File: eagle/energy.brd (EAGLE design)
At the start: 51.7 x 57.8 mm, 19 parts, among them J1 S0, J2 NPN, T1 BC547, X1 P1

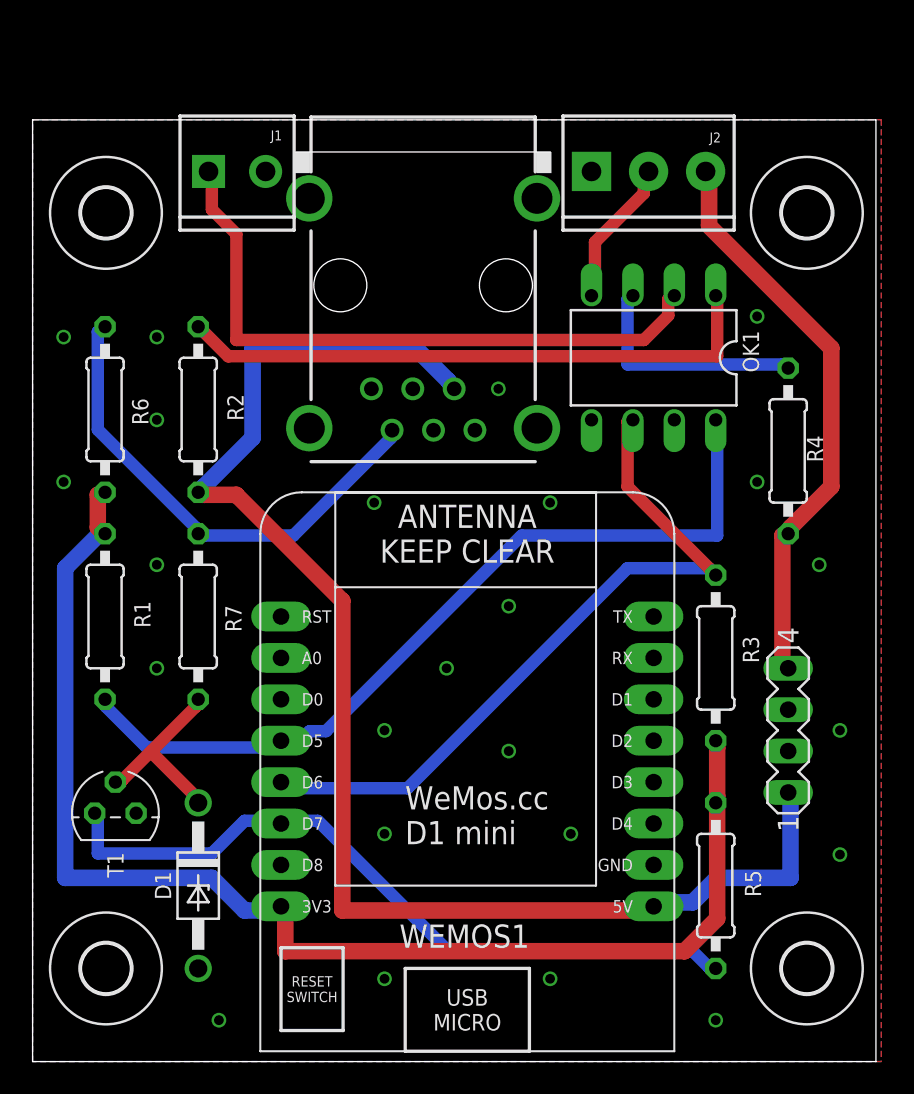
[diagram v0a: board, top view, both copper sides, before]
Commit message: Adjusted PCB
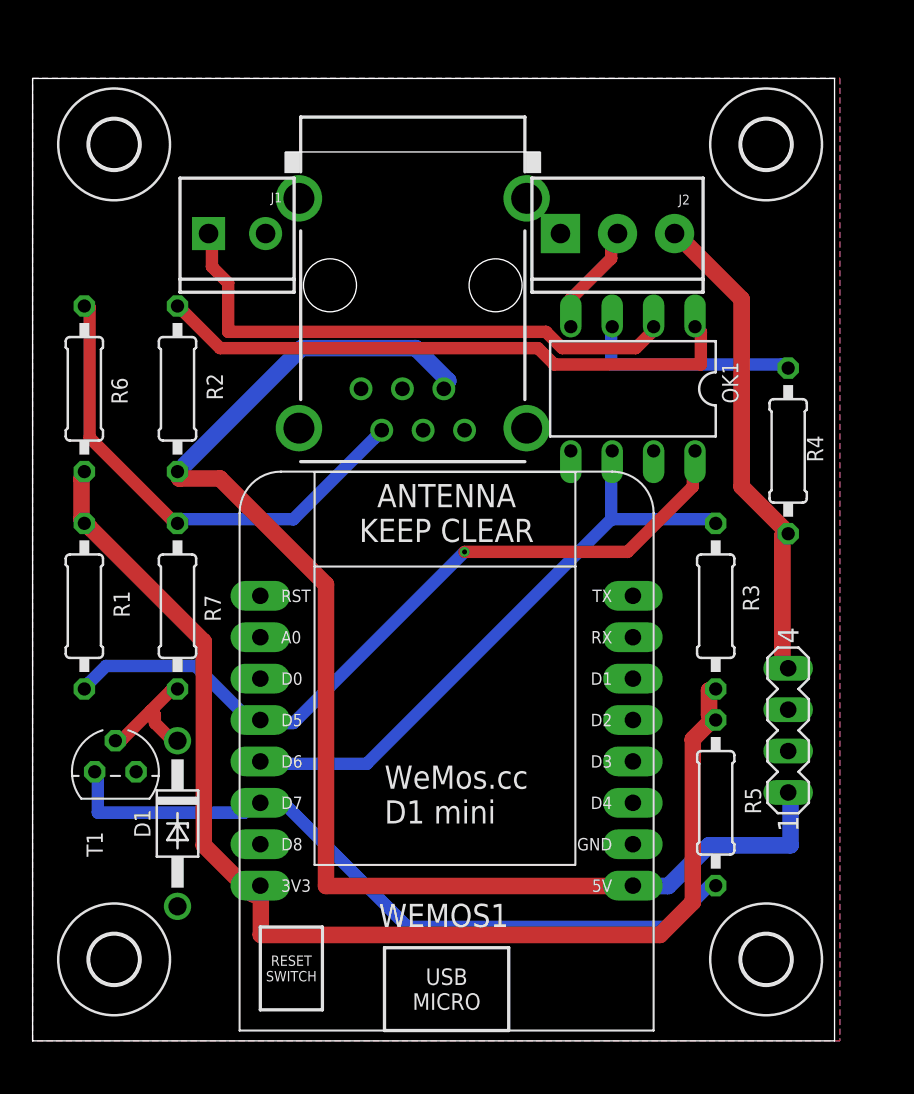
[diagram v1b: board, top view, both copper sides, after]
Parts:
- moved R5 5.08 mm to (41.9, 14.6)
- moved H4 4.89 mm to (45.0, 55.0)
- moved J2 4.26 mm to (32.4, 49.5)
- moved H3 4.23 mm to (5.00, 55.0)
- moved D1 4.02 mm to (8.89, 13.3)
- moved J1 3.81 mm to (10.8, 49.5)
- moved R3 3.18 mm to (41.9, 26.7)
- moved H1 2.56 mm to (45.0, 5.00)
- moved T1 2.54 mm to (5.08, 16.5)
- moved OK1 2.29 mm to (36.8, 40.0)
- moved R6 1.80 mm to (3.17, 40.0)
- moved R2 1.80 mm to (8.89, 40.0)
- moved WEMOS1 1.80 mm to (24.1, 19.7)
- moved R1 1.42 mm to (3.17, 26.7)
- moved R7 1.42 mm to (8.89, 26.7)
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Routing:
- net D6: track 44.6 -> 38.5 mm
- net N$2: track 39.6 -> 33.8 mm
- net 12V: track 35.2 -> 30.1 mm
- net 3V3: track 80.7 -> 75.7 mm
- net D5: track 51.6 -> 47.7 mm, vias 0 -> 1
- net N$1: track 11.6 -> 7.74 mm
- net 5V: track 87.9 -> 84.6 mm
- net NPNOUT: track 9.04 -> 7.11 mm
- net N$3: track 14.3 -> 13.2 mm
- net N$4: track 30.3 -> 30.8 mm
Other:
- board size 51.7 x 57.8 mm -> 49.2 x 59 mm

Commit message: Cleaning up
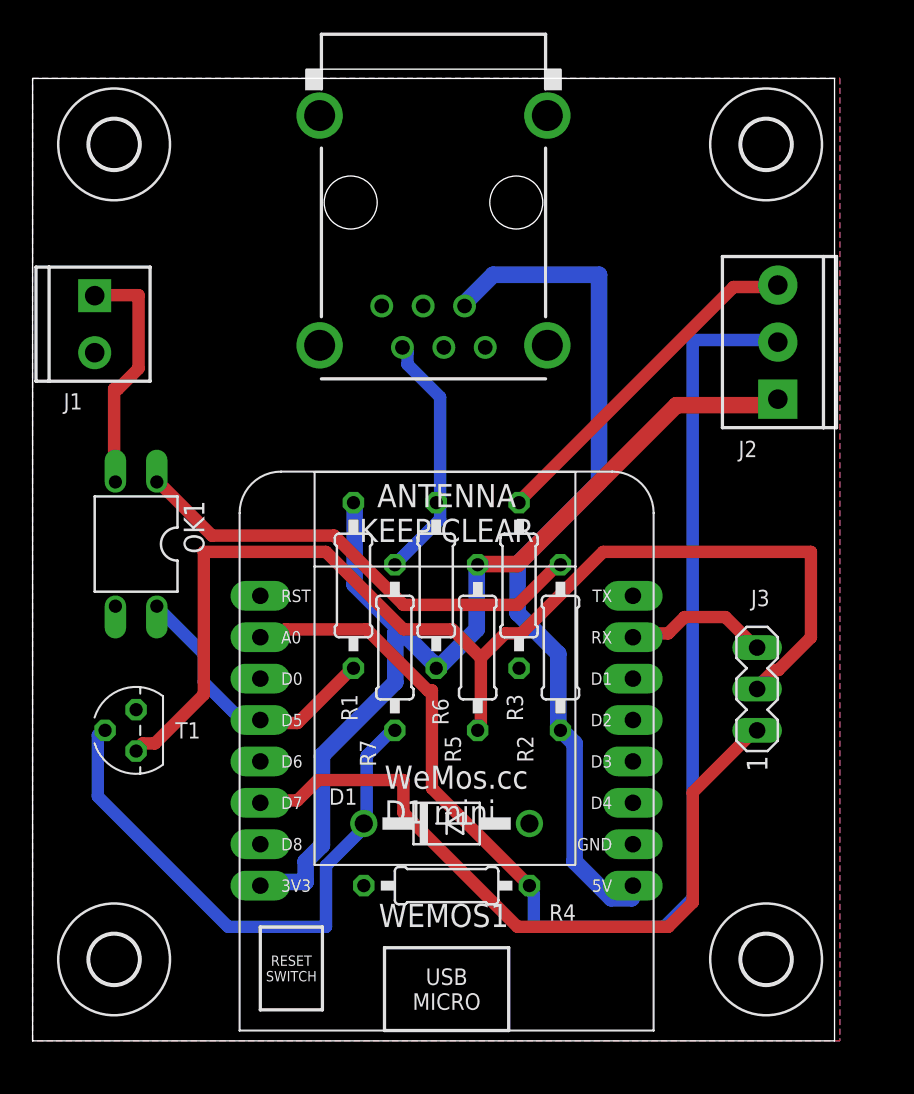
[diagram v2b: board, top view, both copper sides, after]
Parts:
- removed 5VTO12V: STEPUP, con-lstb:MA04-1
- added J3: D7 SEL RX, con-lstb:MA03-1
- J2: value NPN -> OPT
- OK1: value PC827 -> PC817; device optocoupler:DIL08 -> optocoupler:DIL04
- R3: value 4k7 -> 220R
- R4: value 470R -> 4k7
- moved R4 33.9 mm to (25.4, 9.53), turned to 0 degrees
- moved OK1 31.9 mm to (6.35, 30.5)
- moved R2 28.4 mm to (32.4, 24.1)
- moved R6 24.7 mm to (24.8, 27.9)
- moved R5 17.4 mm to (27.3, 24.1)
- moved J2 16.8 mm to (45.7, 39.4), turned to 90 degrees
- moved R1 16.6 mm to (19.7, 27.9)
- moved D1 16.5 mm to (25.4, 13.3), turned to 0 degrees
- moved R7 13.6 mm to (22.2, 24.1)
- moved R3 12.1 mm to (29.8, 27.9), turned to 90 degrees
- moved J1 7.96 mm to (3.81, 45.7), turned to 270 degrees
- moved X1 5.24 mm to (24.6, 51.4)
- moved T1 2.84 mm to (6.35, 19.1), turned to 90 degrees
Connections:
- removed net 12V: 5VTO12V.4, J2.3, R4.1
- removed net D6: OK1.6, R3.1, WEMOS1.D6
- new net N$5: J3.1, WEMOS1.D7
- new net N$6: J3.3, WEMOS1.RX
- net 3V3: now also J2.1; no longer R3.2
- net 5V: no longer 5VTO12V.1
- net D5: now also OK1.4; no longer OK1.8
- net D7: now also J3.2; no longer WEMOS1.D7
- net GND: now also OK1.3, R3.1, R4.1; no longer 5VTO12V.2, 5VTO12V.3, J2.1, OK1.5, OK1.7
- net N$3: now also J2.3, R3.2; no longer OK1.3, R4.2
- net NPNOUT: now also R4.2, WEMOS1.A0; no longer OK1.4
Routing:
- net NPNOUT: track 7.11 -> 79.4 mm
- net N$5: track 0.00 -> 44.9 mm
- net D6: track 38.5 -> 0.00 mm
- net 5V: track 84.6 -> 53.9 mm
- net D5: track 47.7 -> 17.5 mm, vias 1 -> 0
- net 12V: track 30.1 -> 0.00 mm
- net N$1: track 7.74 -> 35.5 mm
- net D7: track 45.0 -> 71.4 mm
- net N$2: track 33.8 -> 14.9 mm
- net N$4: track 30.8 -> 15.8 mm
- net 3V3: track 75.7 -> 63.1 mm
- net N$6: track 0.00 -> 8.91 mm
- net N$3: track 13.2 -> 21.4 mm
- net N$8: track 36.1 -> 28.9 mm
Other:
- board text added: "Utility Shield v0.4"
- board text removed: "Utility Shield v0.3"
